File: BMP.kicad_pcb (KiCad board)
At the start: 2 copper layers, 67.5 x 31.5 mm, 35 parts, among them CN1 USB_B_Mini, J1 Conn_01x04_Pin, J2 Conn_02x05_Odd_Even, Q1 IRLML5203, SW1 SW_Push, SW2 SW_Push, U1 STM32F103CBTx, U2 TXS0108EPW, U3 TLV70033_SOT23-5, Y1 8MHz

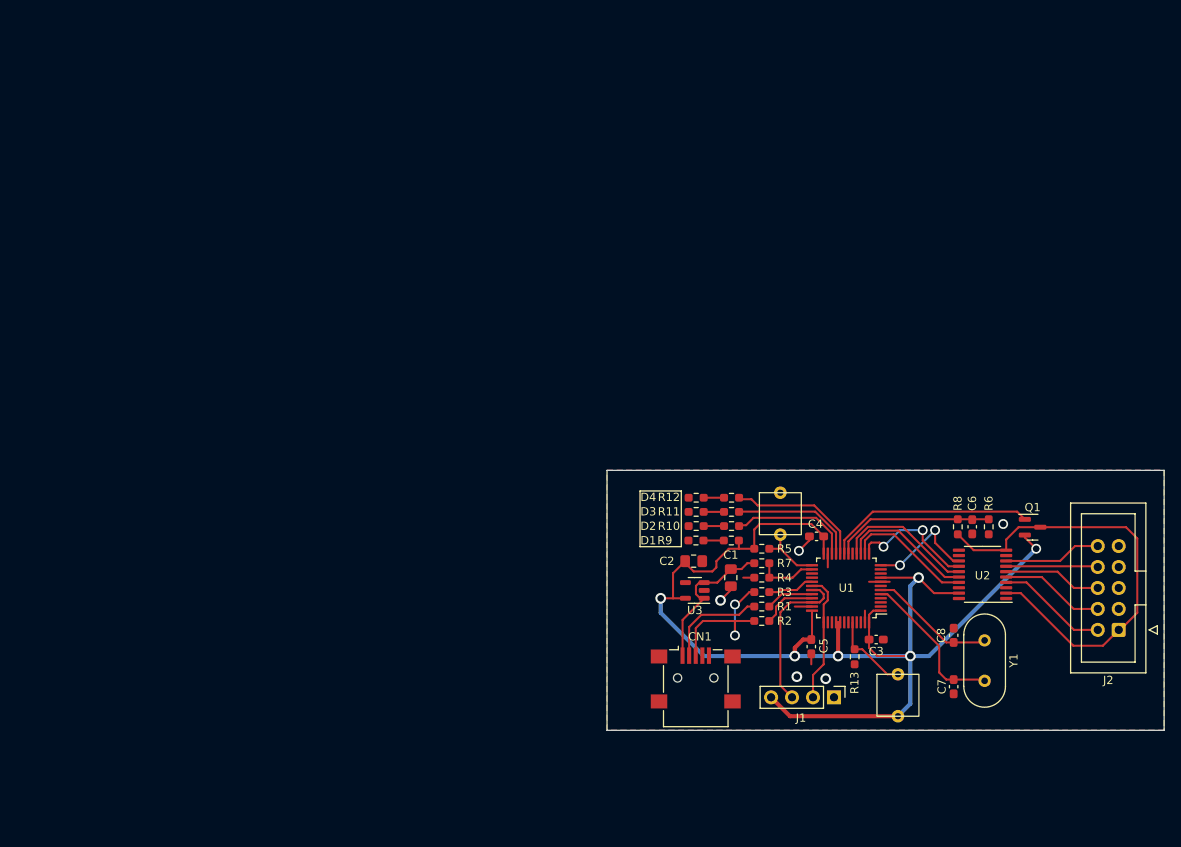
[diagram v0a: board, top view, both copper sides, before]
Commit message: 17032023
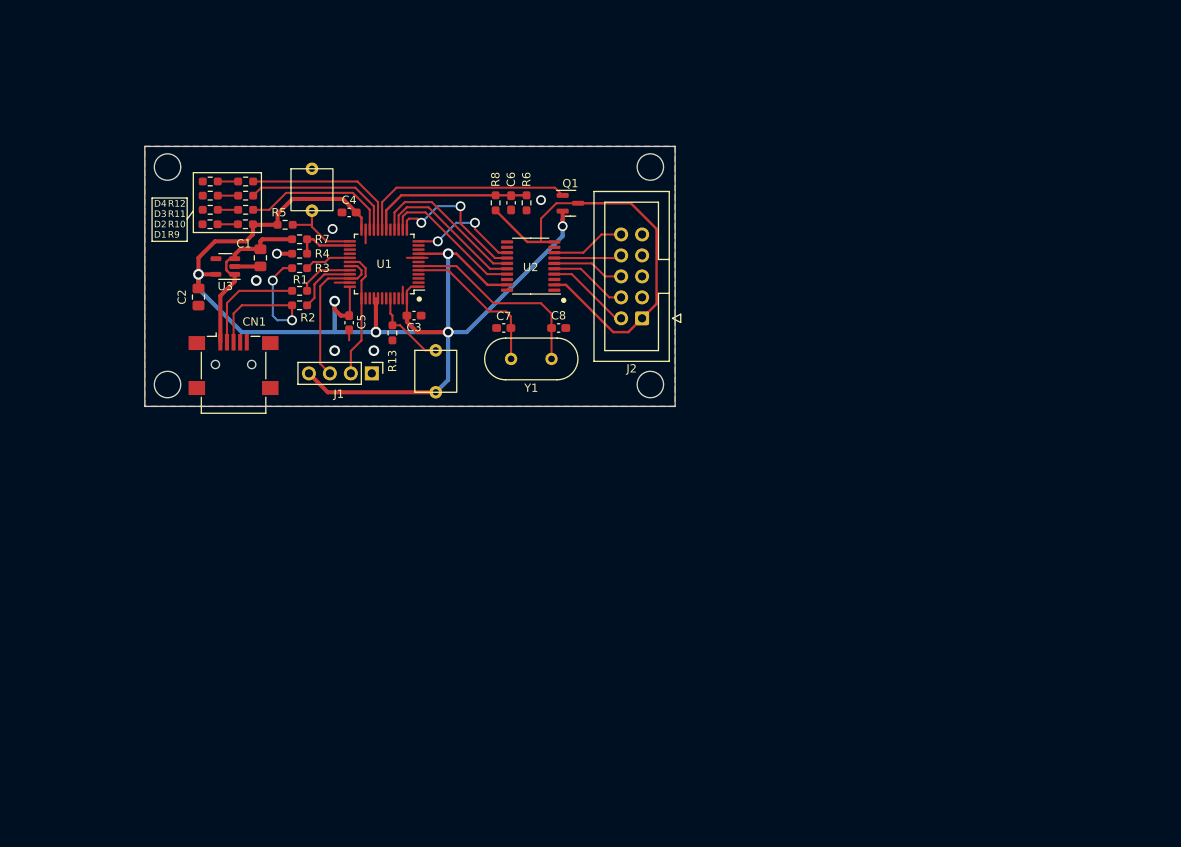
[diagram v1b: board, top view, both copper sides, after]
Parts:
- moved D1 70.2 mm to (25.4, 25.9)
- moved D2 70.2 mm to (25.4, 24.2)
- moved D3 70.2 mm to (25.4, 22.5)
- moved D4 70.2 mm to (25.4, 20.8)
- moved R10 70.2 mm to (29.7, 24.2)
- moved R11 70.2 mm to (29.7, 22.5)
- moved R12 70.2 mm to (29.7, 20.8)
- moved R9 70.2 mm to (29.7, 25.9)
- moved R5 69.8 mm to (34.5, 26.0)
- moved C7 69.7 mm to (61.0, 38.5), turned to 0 degrees
- moved U3 69.1 mm to (27.2, 31.1)
- moved SW1 69.0 mm to (37.8, 21.8)
- moved J2 69.0 mm to (77.8, 37.3)
- moved C1 68.9 mm to (31.5, 30.0)
- moved C4 68.9 mm to (42.2, 24.5)
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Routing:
- net Net-(U1-PD1): track 15.3 -> 24.0 mm
- net /LED2: track 14.7 -> 18.2 mm
- net Net-(CN1-D+): track 19.2 -> 22.7 mm
- net /LED1: track 15.4 -> 18.8 mm
- net /TARGET_TCK: track 12.7 -> 9.53 mm
- net /TARGET_TDO: track 11.9 -> 8.75 mm
- net /TARGET_TMS: track 13.5 -> 10.3 mm
- net /TARGET_TDI: track 11.1 -> 8.23 mm
- net /LED0: track 16.6 -> 19.5 mm
- net /TARGET_RST: track 11.8 -> 9.01 mm
- net /TDI: track 15.7 -> 18.2 mm
- net +3.3V: track 157.4 -> 159.6 mm
- net /TDO: track 17.1 -> 19.3 mm
- net /TCK: track 16.4 -> 18.4 mm
- net /FORCE_BOOTLOADER: track 7.71 -> 9.61 mm
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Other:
- board size 67.5 x 31.5 mm -> 64.2 x 31.5 mm

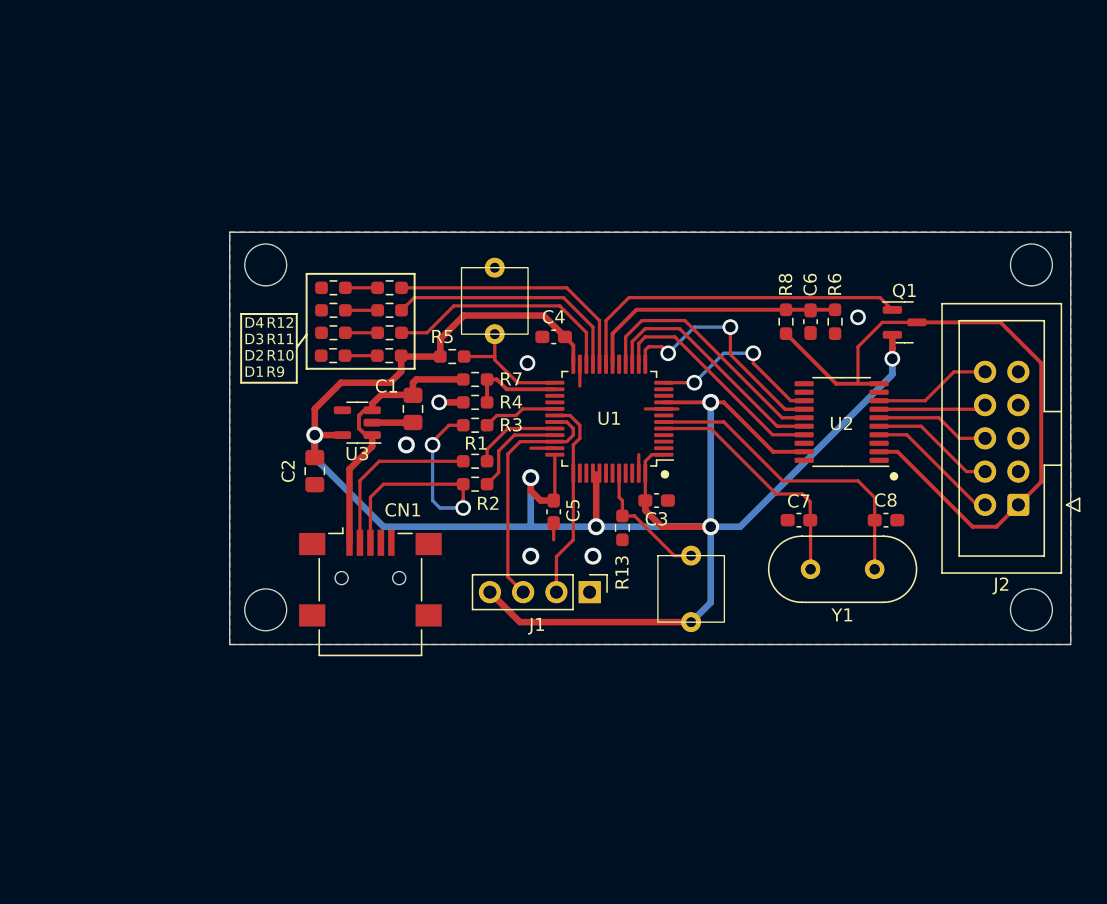
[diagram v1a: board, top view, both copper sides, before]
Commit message: 18032022
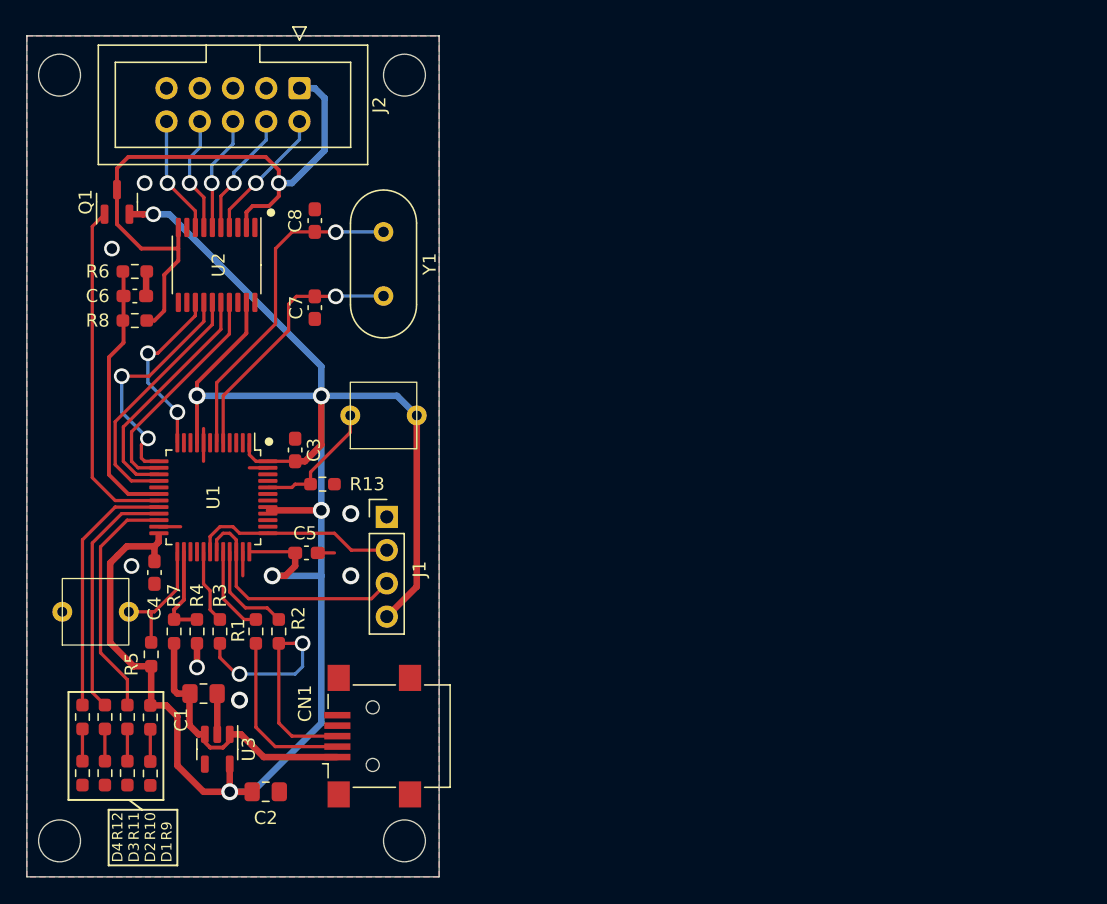
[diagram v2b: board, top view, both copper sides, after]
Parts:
- moved J2 63.5 mm to (22.8, 5.50), turned to -90 degrees
- moved Q1 60.9 mm to (8.89, 14.2), turned to 90 degrees
- moved R6 53.6 mm to (10.2, 19.5), turned to 180 degrees
- moved C6 51.7 mm to (10.2, 21.4), turned to 180 degrees
- moved R8 49.8 mm to (10.2, 23.2), turned to 180 degrees
- moved C8 49.3 mm to (24.0, 15.6), turned to -90 degrees
- moved U2 49.2 mm to (16.5, 19.0), turned to -90 degrees
- moved Y1 45.5 mm to (29.2, 16.5), turned to -90 degrees
- moved D4 41.7 mm to (6.25, 57.8), turned to 90 degrees
- moved C7 40.4 mm to (24.0, 22.3), turned to 90 degrees
- moved R12 40.3 mm to (6.25, 53.5), turned to -90 degrees
- moved D3 39.4 mm to (7.97, 57.8), turned to 90 degrees
- moved SW1 38.7 mm to (7.25, 45.5), turned to 0 degrees
- moved R11 37.9 mm to (7.97, 53.5), turned to -90 degrees
- moved D2 37.1 mm to (9.68, 57.8), turned to 90 degrees
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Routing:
- net /TPWR: track 52.8 -> 48.2 mm, vias 0 -> 1
- net GND: track 14.0 -> 15.9 mm, vias 6 -> 7
- net Net-(U1-PD0): track 18.7 -> 20.2 mm, vias 0 -> 1
- net Net-(U1-PD1): track 24.0 -> 25.4 mm, vias 0 -> 1
- net +3.3V: track 159.6 -> 161.0 mm
- net /TARGET_TDI: track 8.23 -> 8.90 mm, vias 0 -> 1
- net /TARGET_TDO: track 8.75 -> 8.79 mm, vias 0 -> 1
- net /TARGET_TCK: vias 0 -> 1
- net /TARGET_TMS: vias 0 -> 1
- net /TARGET_RST: vias 0 -> 1
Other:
- board size 64.2 x 31.5 mm -> 31.5 x 64.2 mm

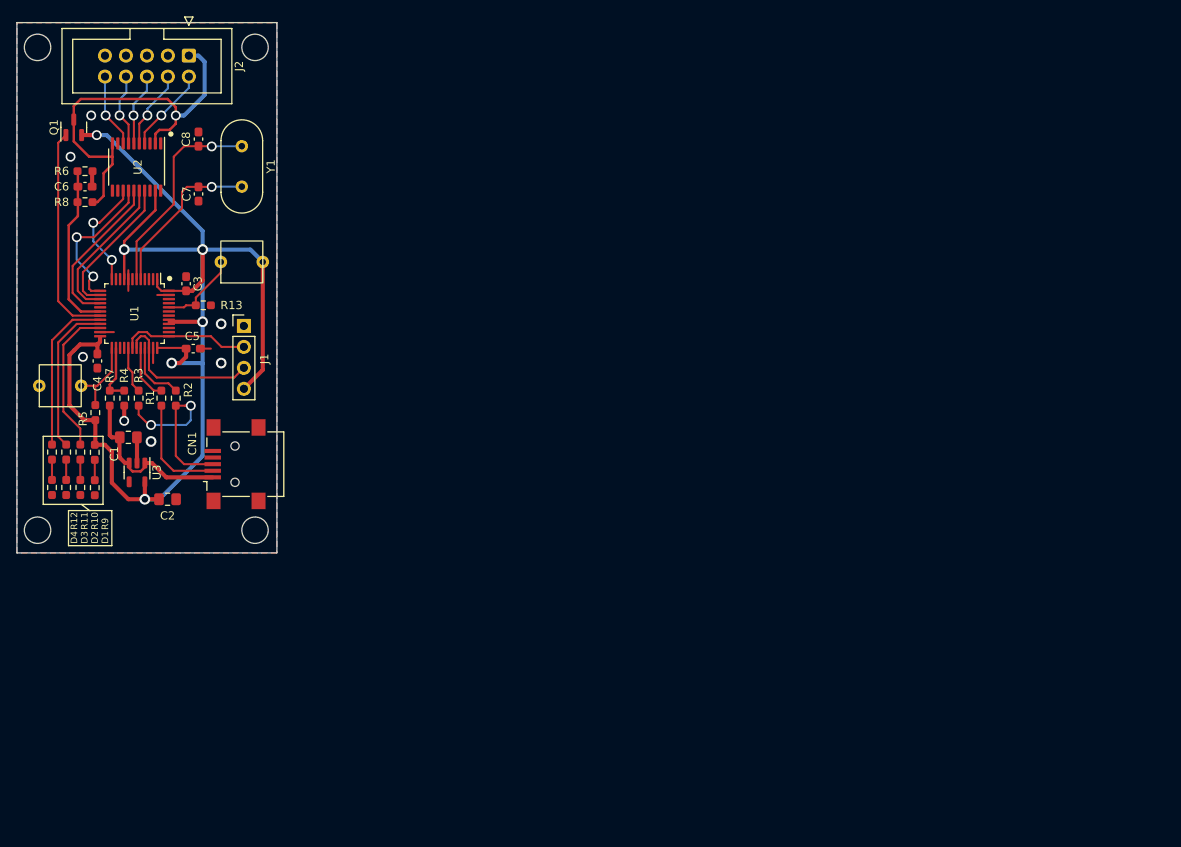
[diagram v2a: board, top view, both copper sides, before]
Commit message: 29042023
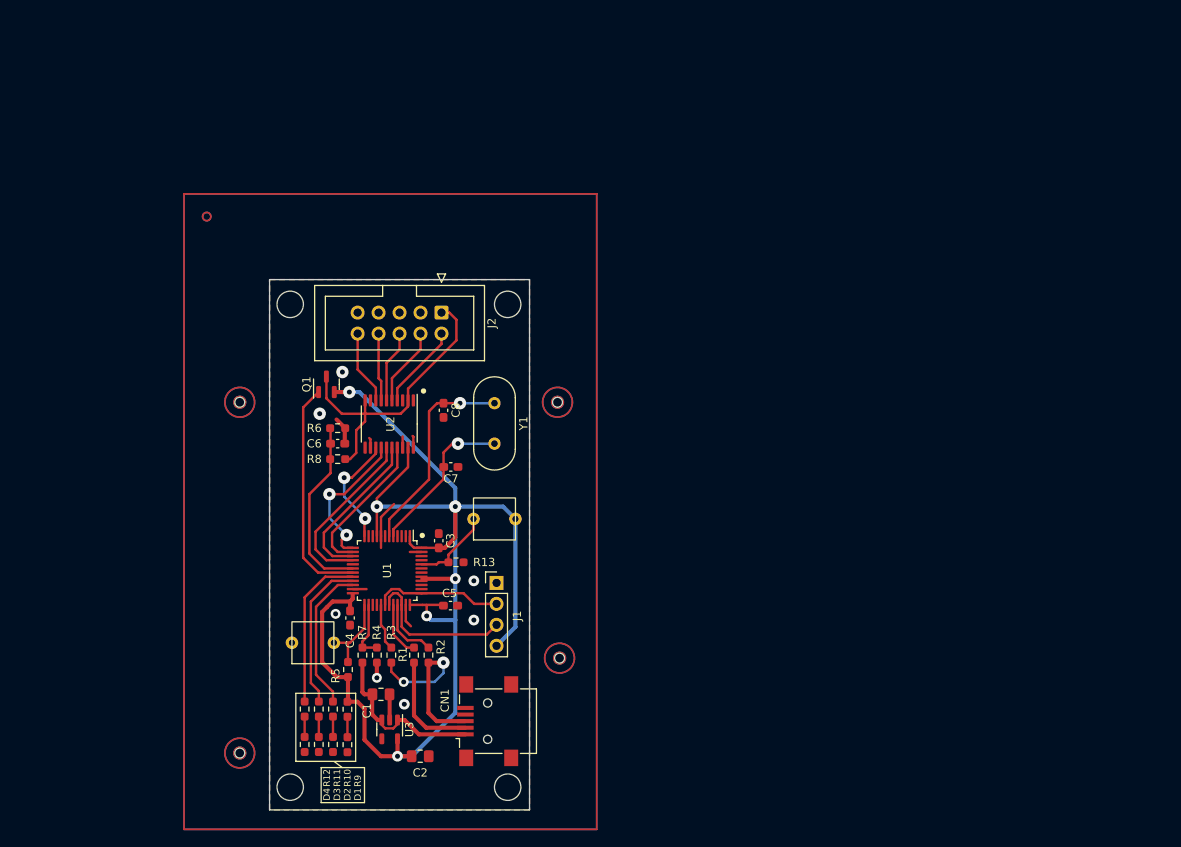
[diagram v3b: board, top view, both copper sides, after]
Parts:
- added REF**: reper, Custom PADs:reper, F.Cu at (29.0, 47.5)
- added REF**: reper, Custom PADs:reper, F.Cu at (67.8, 78.5)
- added REF**: reper, Custom PADs:reper, F.Cu at (67.5, 47.5)
- added REF**: reper, Custom PADs:reper, F.Cu at (29.0, 90.0)
- moved C7 45.0 mm to (54.6, 55.3), turned to 180 degrees
- moved C8 44.3 mm to (53.7, 48.5), turned to 90 degrees
- moved C5 44.1 mm to (54.5, 72.1)
- moved CN1 43.7 mm to (59.0, 86.1)
- moved D3 43.7 mm to (38.6, 89.0)
- moved J2 43.7 mm to (53.4, 36.6)
- moved Q1 43.7 mm to (39.5, 45.3)
- moved R13 43.7 mm to (55.2, 66.9)
- moved U3 43.7 mm to (47.2, 87.1)
- moved C1 43.7 mm to (46.1, 82.9)
- moved C2 43.7 mm to (50.9, 90.4)
- moved C3 43.7 mm to (53.1, 64.3)
- moved C4 43.7 mm to (42.4, 73.6)
- moved C6 43.7 mm to (40.9, 52.5)
- moved D1 43.7 mm to (42.0, 89.0)
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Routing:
- net /TPWR: track 48.2 -> 37.2 mm, vias 1 -> 0
- net GND: track 15.9 -> 24.6 mm
- net /TARGET_POWER_ADC: track 20.4 -> 22.3 mm
- net /TDO: track 19.3 -> 21.0 mm
- net /PWR_BR: track 26.3 -> 27.6 mm
- net +3.3V: track 161.0 -> 159.7 mm
- net /TCK: track 18.4 -> 19.5 mm
- net Net-(U1-PD0): track 20.2 -> 19.3 mm
- net /TARGET_TDI: track 8.90 -> 8.23 mm, vias 1 -> 0
- net /TARGET_TDO: track 8.79 -> 8.75 mm, vias 1 -> 0
- net /TARGET_RST: vias 1 -> 0
- net /TARGET_TCK: vias 1 -> 0
- net /TARGET_TMS: vias 1 -> 0
